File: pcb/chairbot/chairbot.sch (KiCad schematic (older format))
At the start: 18 parts, among them J1 Conn_01x02, J2 Conn_01x05, U1 ESP32mini, U2 74HCT08, U3 74HCT244, U4 buck-converter, U5 nRF24L01+, U8 AMS1117-3.3, U9 PCA9515

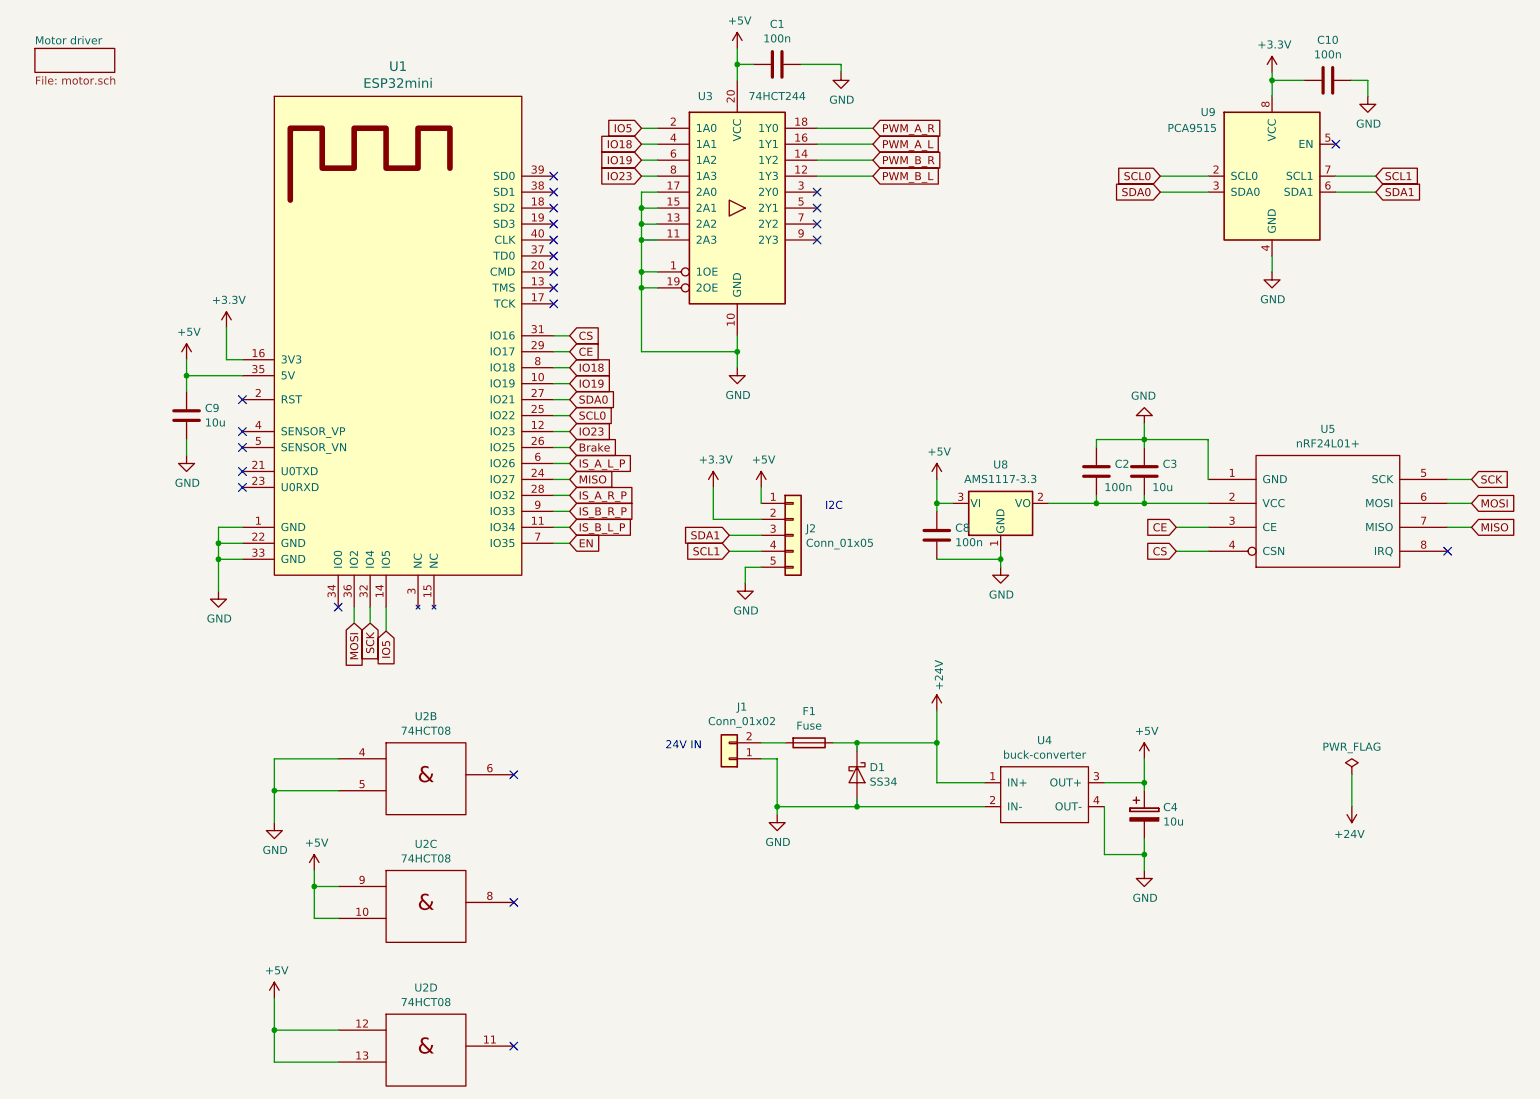
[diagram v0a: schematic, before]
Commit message: Fix various issues.
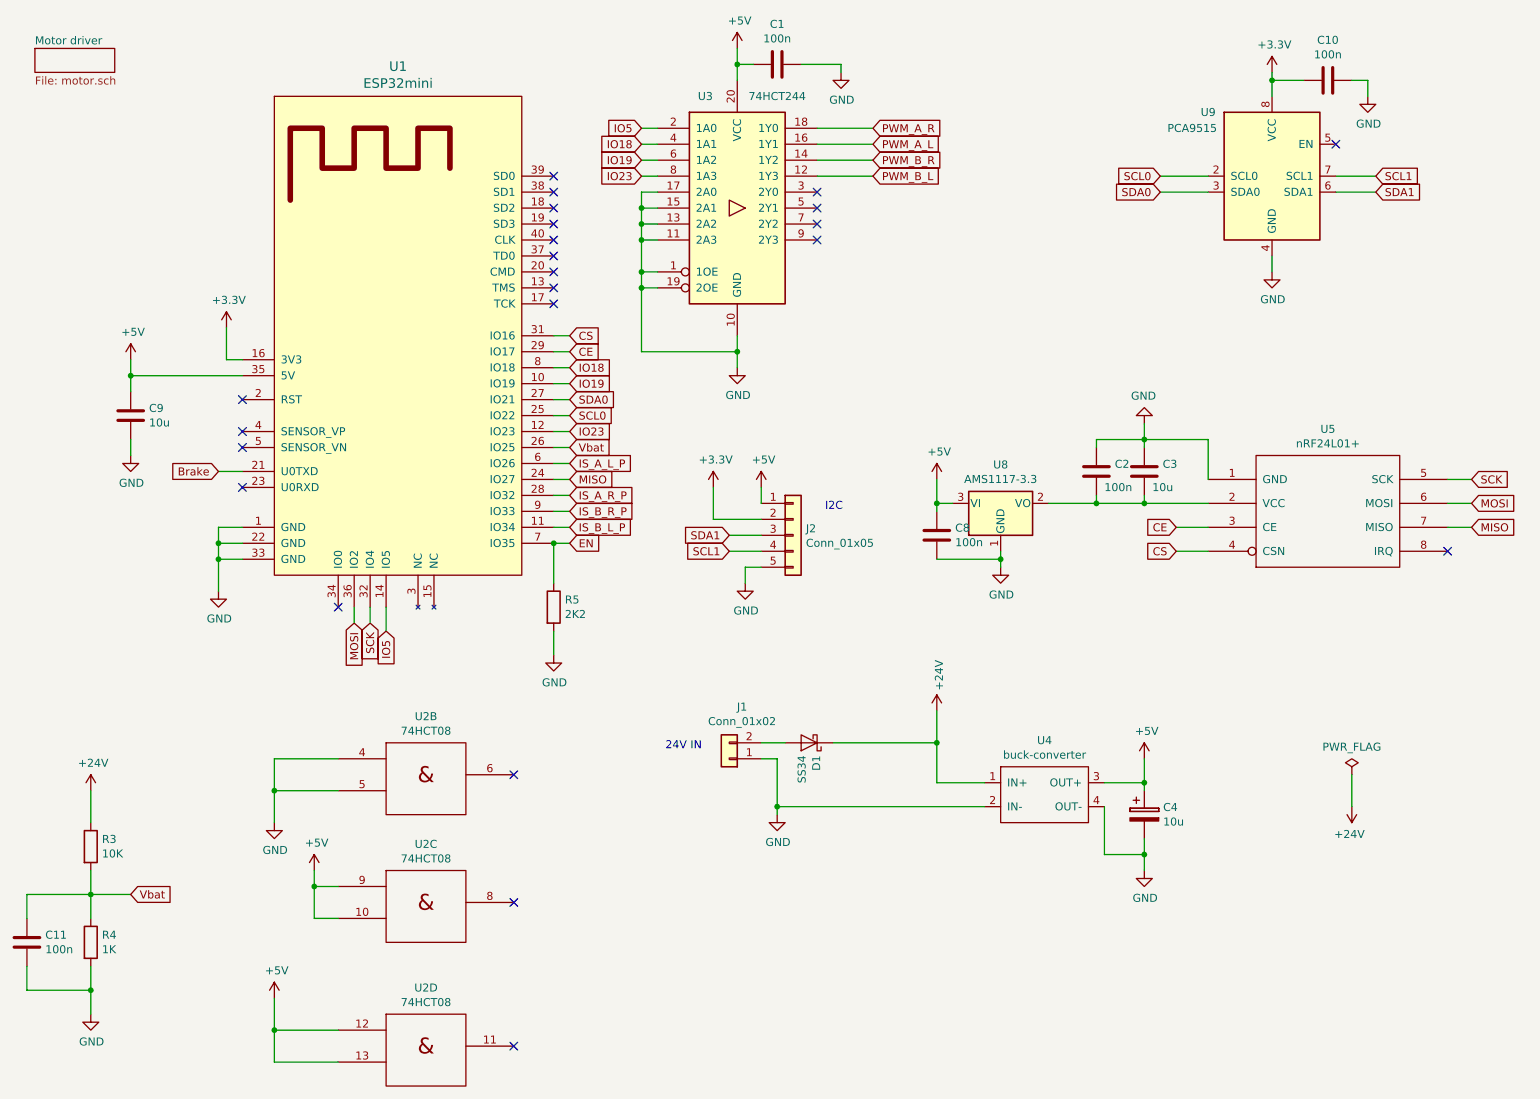
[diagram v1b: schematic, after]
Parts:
- removed F1: Fuse, Resistor_THT:R_Axial_DIN0309_L9.0mm_D3.2mm_P2.54mm_Vertical, symbol Device:Fuse
- added C11: 100n, Capacitor_SMD:C_0603_1608Metric, symbol Device:C
- added R3: 10K, Resistor_SMD:R_0603_1608Metric, symbol Device:R
- added R4: 1K, Resistor_SMD:R_0603_1608Metric, symbol Device:R
- added R5: 2K2, Resistor_SMD:R_0603_1608Metric, symbol Device:R
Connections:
- net +24V: now also R3.1
- net Brake: now also U1.21 (U0TXD); no longer U1.26 (IO25)
- net EN: now also R5.1
- net GND: now also C11.2, R4.2, R5.2; no longer D1.2 (A)
- net at J1.2 (Pin_2): now also D1.2 (A)
- new net Vbat: C11.1, R3.2, R4.1, U1.26 (IO25)
- no-connect marks 24 -> 23
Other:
- moved on the sheet: C9, D1
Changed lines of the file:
@@
 	5450 5350 5550 5350
 $Comp
-L Device:Fuse F1
-U 1 1 5BD26A01
+L Device:D_Schottky D1
+U 1 1 5BD26B72
 P 5750 5250
-F 0 "F1" V 5553 5250 50  0000 C CNN
-F 1 "Fuse" V 5644 5250 50  0000 C CNN
-F 2 "Resistor_THT:R_Axial_DIN0309_L9.0mm_D3.2mm_P2.54mm_Vertical" V 5680 5250 50  0001 C CNN
+F 0 "D1" V 5704 5329 50  0000 L CNN
+F 1 "SS34" V 5795 5329 50  0000 L CNN
+F 2 "Diode_SMD:D_SMB" H 5750 5250 50  0001 C CNN
 F 3 "~" H 5750 5250 50  0001 C CNN
 	1    5750 5250
-	0    1    1    0
-$EndComp
-$Comp
-L Device:D_Schottky D1
-U 1 1 5BD26B72
-P 6050 5450
-F 0 "D1" V 6004 5529 50  0000 L CNN
-F 1 "SS34" V 6095 5529 50  0000 L CNN
-F 2 "Diode_SMD:D_SMB" H 6050 5450 50  0001 C CNN
-F 3 "~" H 6050 5450 50  0001 C CNN
-	1    6050 5450
-	0    1    1    0
+	-1   0    0    1
 $EndComp
 Wire Wire Line
 	5550 5350 5550 5650
-Wire Wire Line
-	6050 5600 6050 5650
-Wire Wire Line
-	6050 5650 5550 5650
 Connection ~ 5550 5650
 Wire Wire Line
@@
 Wire Wire Line
 	5450 5250 5600 5250
-Wire Wire Line
-	5900 5250 6050 5250
-Wire Wire Line
-	6050 5250 6050 5300
 $Comp
 L power:+24V #PWR03
@@
 	1    0    0    -1
 $EndComp
-Connection ~ 6050 5250
 $Comp
 L buckconverter:buck-converter U4
@@
 	6550 5500 6850 5500
 Wire Wire Line
-	6050 5250 6550 5250
-Wire Wire Line
 	6550 5050 6550 5250
 Connection ~ 6550 5250
-Wire Wire Line
-	6050 5650 6850 5650
-Connection ~ 6050 5650
 $Comp
 L power:+5V #PWR06
@@
 Text GLabel 4250 4000 2    50   Input ~ 0
 EN
-Text GLabel 4250 3400 2    50   Input ~ 0
+Text GLabel 2050 3550 0    50   Input ~ 0
 Brake
 $Comp
@@
 L Device:C C9
 U 1 1 5BD55B4E
-P 1850 3200
-F 0 "C9" H 1965 3246 50  0000 L CNN
-F 1 "10u" H 1965 3155 50  0000 L CNN
-F 2 "Capacitor_SMD:C_0805_2012Metric" H 1888 3050 50  0001 C CNN
-F 3 "~" H 1850 3200 50  0001 C CNN
-	1    1850 3200
+P 1500 3200
+F 0 "C9" H 1615 3246 50  0000 L CNN
+F 1 "10u" H 1615 3155 50  0000 L CNN
+F 2 "Capacitor_SMD:C_0805_2012Metric" H 1538 3050 50  0001 C CNN
+F 3 "~" H 1500 3200 50  0001 C CNN
+	1    1500 3200
 	1    0    0    -1
 $EndComp
@@
 L power:+5V #PWR0122
 U 1 1 5BD55BFD
-P 1850 2850
-F 0 "#PWR0122" H 1850 2700 50  0001 C CNN
-F 1 "+5V" H 1865 3023 50  0000 C CNN
-F 2 "" H 1850 2850 50  0001 C CNN
-F 3 "" H 1850 2850 50  0001 C CNN
-	1    1850 2850
-	1    0    0    -1
-$EndComp
-Wire Wire Line
-	1850 2850 1850 2950
-Wire Wire Line
-	2200 2950 1850 2950
-Connection ~ 1850 2950
-Wire Wire Line
-	1850 2950 1850 3050
+P 1500 2850
+F 0 "#PWR0122" H 1500 2700 50  0001 C CNN
+F 1 "+5V" H 1515 3023 50  0000 C CNN
+F 2 "" H 1500 2850 50  0001 C CNN
+F 3 "" H 1500 2850 50  0001 C CNN
+	1    1500 2850
+	1    0    0    -1
+$EndComp
+Wire Wire Line
+	1500 2850 1500 2950
+Connection ~ 1500 2950
+Wire Wire Line
+	1500 2950 1500 3050
 $Comp
 L power:GND #PWR0123
 U 1 1 5BD59785
-P 1850 3450
-F 0 "#PWR0123" H 1850 3200 50  0001 C CNN
-F 1 "GND" H 1855 3277 50  0000 C CNN
-F 2 "" H 1850 3450 50  0001 C CNN
-F 3 "" H 1850 3450 50  0001 C CNN
-	1    1850 3450
-	1    0    0    -1
-$EndComp
-Wire Wire Line
-	1850 3450 1850 3350
+P 1500 3450
+F 0 "#PWR0123" H 1500 3200 50  0001 C CNN
+F 1 "GND" H 1505 3277 50  0000 C CNN
+F 2 "" H 1500 3450 50  0001 C CNN
+F 3 "" H 1500 3450 50  0001 C CNN
+	1    1500 3450
+	1    0    0    -1
+$EndComp
+Wire Wire Line
+	1500 3450 1500 3350
 $Comp
 L power:+3.3V #PWR0124
@@
 Wire Wire Line
 	4150 3400 4250 3400
-NoConn ~ 2200 3550
 NoConn ~ 2200 3650
 $Comp
@@
 	4250 3600 4150 3600
 NoConn ~ 2800 4400
+Wire Wire Line
+	1500 2950 2200 2950
+Wire Wire Line
+	2050 3550 2200 3550
+Text GLabel 4250 3400 2    50   Input ~ 0
+Vbat
+$Comp
+L Device:R R3
+U 1 1 5CB47065
+P 1250 5900
+F 0 "R3" H 1320 5946 50  0000 L CNN
+F 1 "10K" H 1320 5855 50  0000 L CNN
+F 2 "Resistor_SMD:R_0603_1608Metric" V 1180 5900 50  0001 C CNN
+F 3 "~" H 1250 5900 50  0001 C CNN
+	1    1250 5900
+	1    0    0    -1
+$EndComp
+$Comp
+L Device:R R4
+U 1 1 5CB470D2
+P 1250 6500
+F 0 "R4" H 1320 6546 50  0000 L CNN
+F 1 "1K" H 1320 6455 50  0000 L CNN
+F 2 "Resistor_SMD:R_0603_1608Metric" V 1180 6500 50  0001 C CNN
+F 3 "~" H 1250 6500 50  0001 C CNN
+	1    1250 6500
+	1    0    0    -1
+$EndComp
+$Comp
+L power:+24V #PWR011
+U 1 1 5CB4717B
+P 1250 5550
+F 0 "#PWR011" H 1250 5400 50  0001 C CNN
+F 1 "+24V" H 1265 5723 50  0000 C CNN
+F 2 "" H 1250 5550 50  0001 C CNN
+F 3 "" H 1250 5550 50  0001 C CNN
+	1    1250 5550
+	1    0    0    -1
+$EndComp
+$Comp
+L power:GND #PWR012
+U 1 1 5CB47209
+P 1250 6950
+F 0 "#PWR012" H 1250 6700 50  0001 C CNN
+F 1 "GND" H 1255 6777 50  0000 C CNN
+F 2 "" H 1250 6950 50  0001 C CNN
+F 3 "" H 1250 6950 50  0001 C CNN
+	1    1250 6950
+	1    0    0    -1
+$EndComp
+$Comp
+L Device:C C11
+U 1 1 5CB47282
+P 850 6500
+F 0 "C11" H 965 6546 50  0000 L CNN
+F 1 "100n" H 965 6455 50  0000 L CNN
+F 2 "Capacitor_SMD:C_0603_1608Metric" H 888 6350 50  0001 C CNN
+F 3 "~" H 850 6500 50  0001 C CNN
+	1    850  6500
+	1    0    0    -1
+$EndComp
+Wire Wire Line
+	1250 6050 1250 6200
+Wire Wire Line
+	850  6350 850  6200
+Wire Wire Line
+	850  6200 1250 6200
+Connection ~ 1250 6200
+Wire Wire Line
+	1250 6200 1250 6350
+Wire Wire Line
+	1250 5550 1250 5750
+Wire Wire Line
+	1250 6650 1250 6800
+Wire Wire Line
+	850  6650 850  6800
+Wire Wire Line
+	850  6800 1250 6800
+Connection ~ 1250 6800
+Wire Wire Line
+	1250 6800 1250 6950
+Text GLabel 1500 6200 2    50   Input ~ 0
+Vbat
+Wire Wire Line
+	1500 6200 1250 6200
+$Comp
+L Device:R R5
+U 1 1 5CB60365
+P 4150 4400
+F 0 "R5" H 4220 4446 50  0000 L CNN
+F 1 "2K2" H 4220 4355 50  0000 L CNN
+F 2 "Resistor_SMD:R_0603_1608Metric" V 4080 4400 50  0001 C CNN
+F 3 "~" H 4150 4400 50  0001 C CNN
+	1    4150 4400
+	1    0    0    -1
+$EndComp
+$Comp
+L power:GND #PWR013
+U 1 1 5CB60409
+P 4150 4700
+F 0 "#PWR013" H 4150 4450 50  0001 C CNN
+F 1 "GND" H 4155 4527 50  0000 C CNN
+F 2 "" H 4150 4700 50  0001 C CNN
+F 3 "" H 4150 4700 50  0001 C CNN
+	1    4150 4700
+	1    0    0    -1
+$EndComp
+Wire Wire Line
+	4150 4700 4150 4550
+Wire Wire Line
+	4150 4000 4150 4250
+Connection ~ 4150 4000
+Wire Wire Line
+	5900 5250 6550 5250
+Wire Wire Line
+	5550 5650 6850 5650
 $EndSCHEMATC
